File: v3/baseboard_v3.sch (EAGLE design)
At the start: 41 parts, among them Q1 18A/40V/5mΩ, U1 MC33926, U2 MC33926, U3 Value

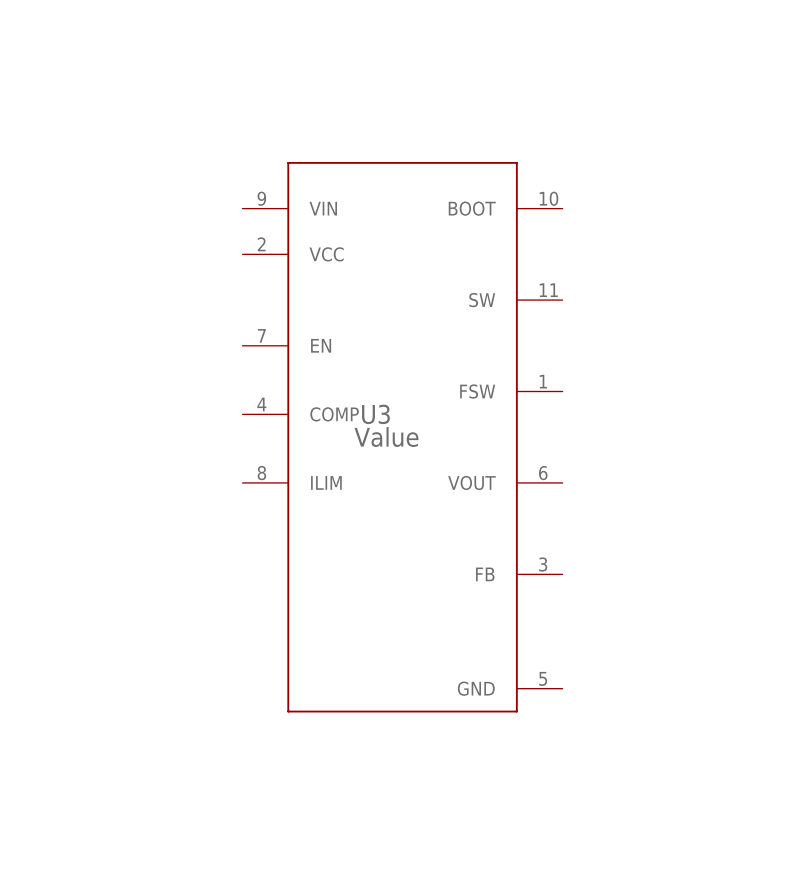
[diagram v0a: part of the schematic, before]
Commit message: Moving away from bb ideas.
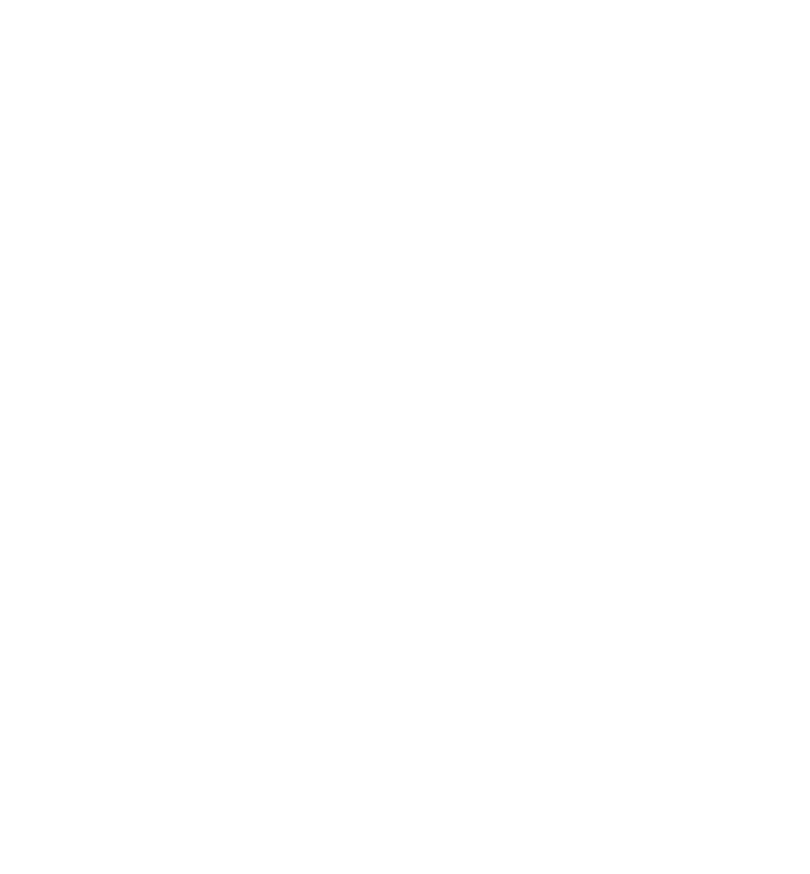
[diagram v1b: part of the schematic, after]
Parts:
- removed U3: Value, powerbench:TPS61089RNRR
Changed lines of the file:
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@@
 <?xml version="1.0" encoding="utf-8"?>
 <!DOCTYPE eagle SYSTEM "eagle.dtd">
-<eagle version="8.0.1">
+<eagle version="8.1.0">
 <drawing>
 <settings>
@@
 <part name="C6" library="SparkFun-Capacitors" deviceset="0.1UF" device="-0603-25V-(+80/-20%)" value="0.1uF"/>
 <part name="SUPPLY18" library="SparkFun-PowerSymbols" deviceset="AGND" device=""/>
-<part name="U3" library="powerbench" deviceset="TPS61089RNRR" device="" value="Value"/>
 </parts>
 <sheets>
@@
 </instance>
 <instance part="SUPPLY18" gate="G$1" x="220.98" y="215.9"/>
-<instance part="U3" gate="A" x="279.4" y="175.26"/>
 </instances>
 <busses>
